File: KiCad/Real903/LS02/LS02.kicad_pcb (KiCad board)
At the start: 2 copper layers, 50.8 x 19 mm, 19 parts, among them J1 Conn_01x06, J2 Conn_01x03, J3 Conn_01x03

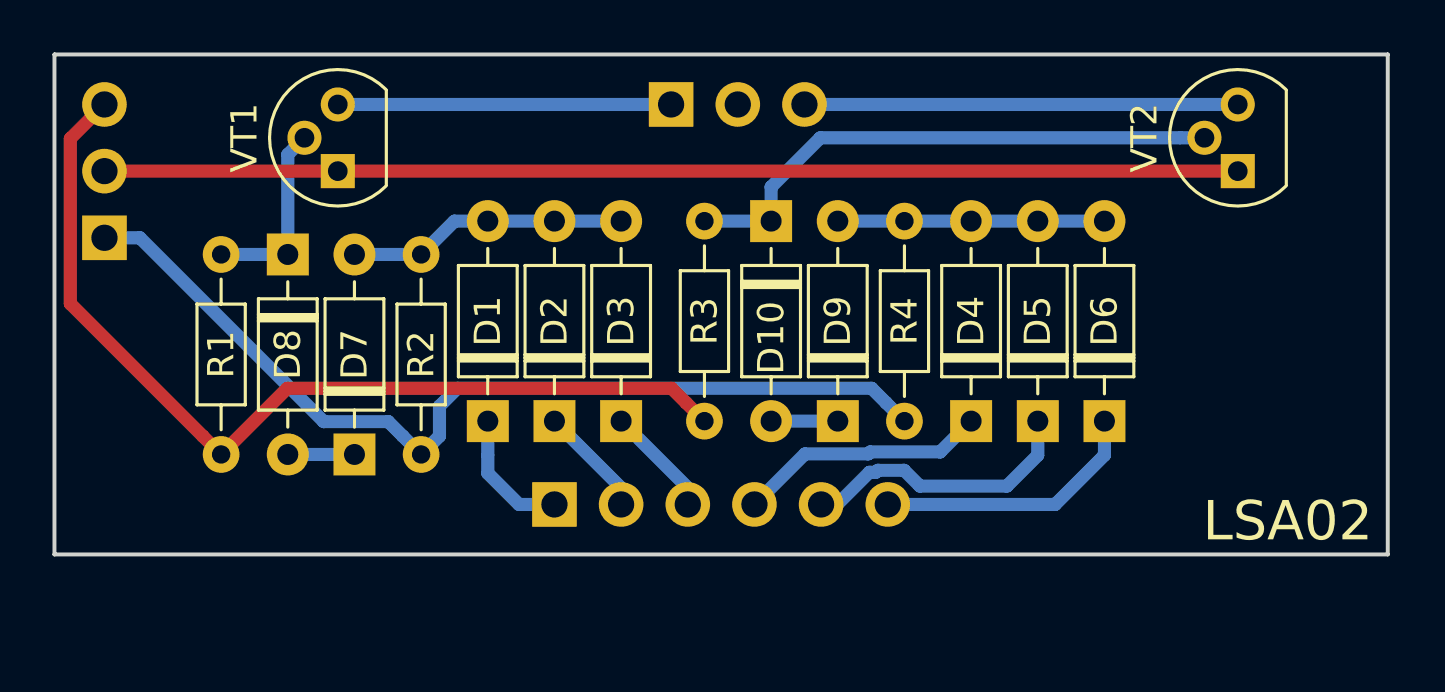
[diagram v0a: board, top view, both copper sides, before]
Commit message: New Kicad design files
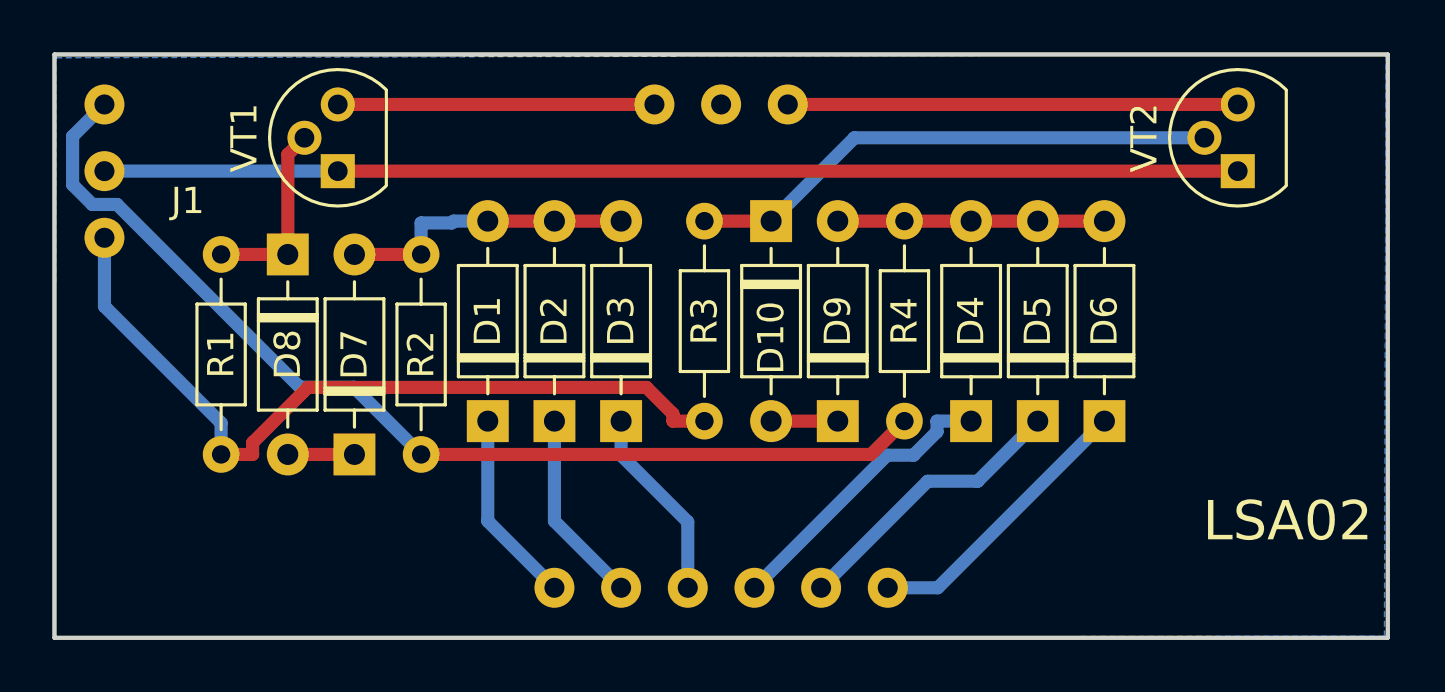
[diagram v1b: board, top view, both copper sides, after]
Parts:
- removed J2, J3: Conn_01x03, ELLIOTT:PinHeader_1x03_P2.54mm_Vertical
- J1: value Conn_01x06 -> LSAConnect; footprint ELLIOTT:PinHeader_1x06_P2.54mm_Vertical -> ELLIOTT:LSA; moved to F.Cu
- moved J1 18.5 mm to (100.3, 43.2), turned to 0 degrees
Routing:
- net -6v: track 36.2 -> 30.5 mm
- net +6v: track 36.1 -> 40.0 mm
- net 3: track 4.23 -> 7.40 mm
- net 2: track 4.23 -> 7.40 mm
- net 1: track 5.02 -> 7.40 mm
- net 4: track 9.57 -> 11.1 mm
- net Net-(D10-Pad1): track 21.1 -> 20.4 mm
- net Net-(D1-Pad2): track 10.7 -> 11.4 mm
- net 13: track 16.5 -> 17.1 mm
- net 11: track 12.7 -> 12.1 mm
- net 6: track 10.3 -> 10.9 mm
- added copper zone on B.Cu, net 0v
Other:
- board size 50.8 x 19 mm -> 50.8 x 22.2 mm
